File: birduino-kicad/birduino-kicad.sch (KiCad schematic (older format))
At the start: 28 parts, among them J1 Conn_01x03_Male, J10 Conn_01x01_Male, J2 Conn_01x02_Male, J3 Conn_02x05_Odd_Even, J4 Conn_01x04, J5 Conn_01x01_Male, J6 Conn_01x01_Male, J7 Conn_01x01_Male, J8 Conn_02x02_Odd_Even, J9 Conn_01x02, Q1 2N7000, Q2 2N7000, Q3 2N7000, SW1 SW_Push_Dual, SW2 SW_Push_Dual, SW3 SW_Push_Dual, SW4 SW_Push_Dual, U1 ATMEGA328-PU, U2 DS18B20

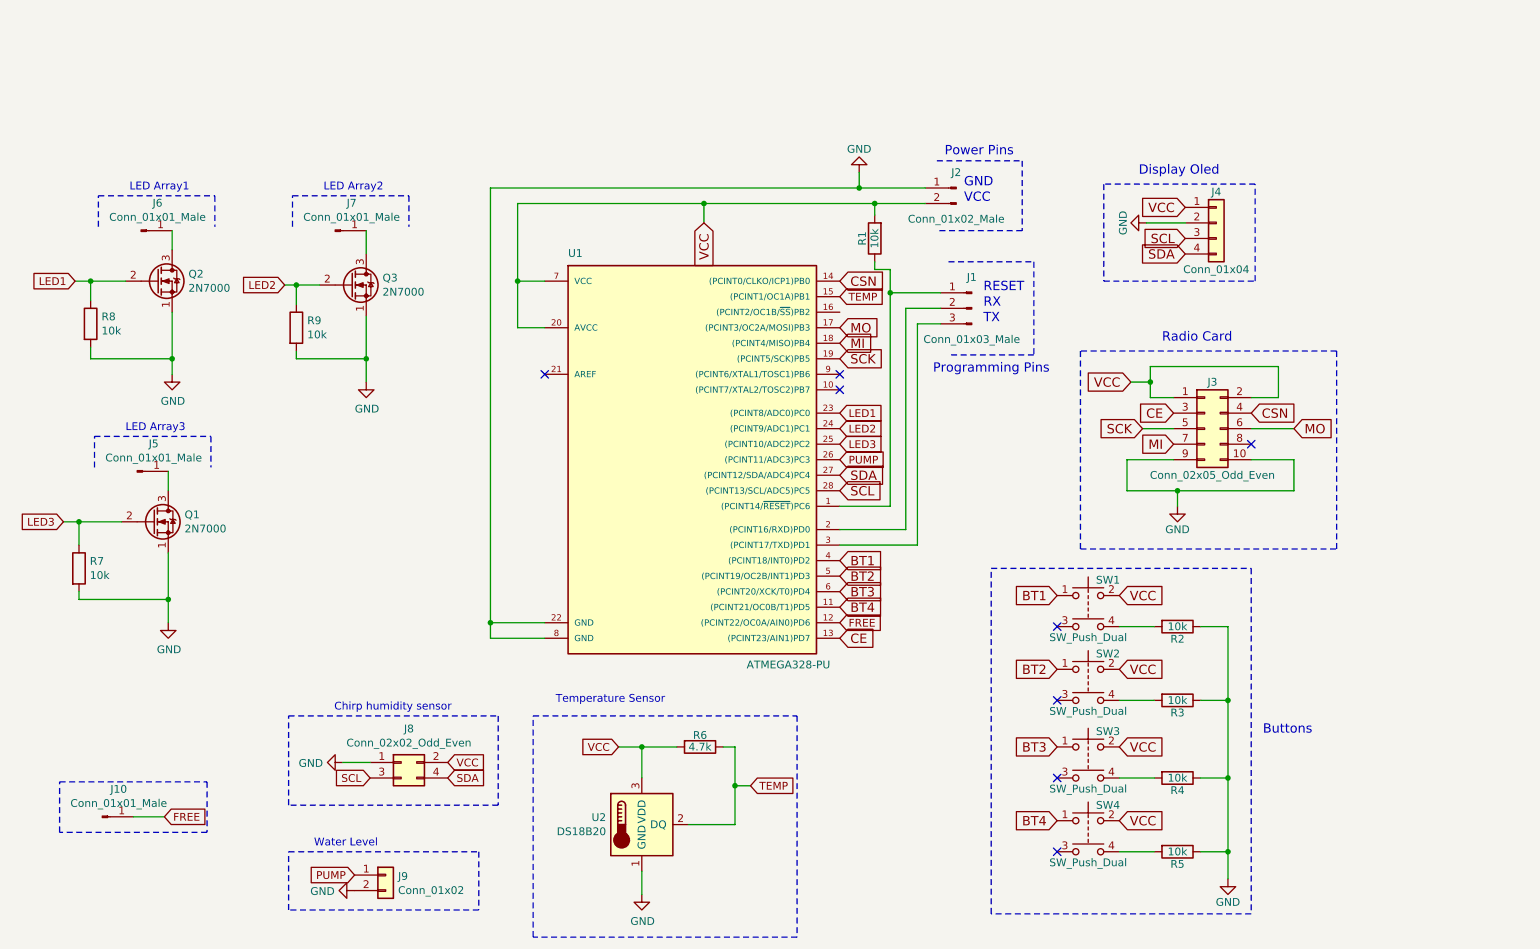
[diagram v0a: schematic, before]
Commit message: feat: First final version 1.0. 3D image added to readme
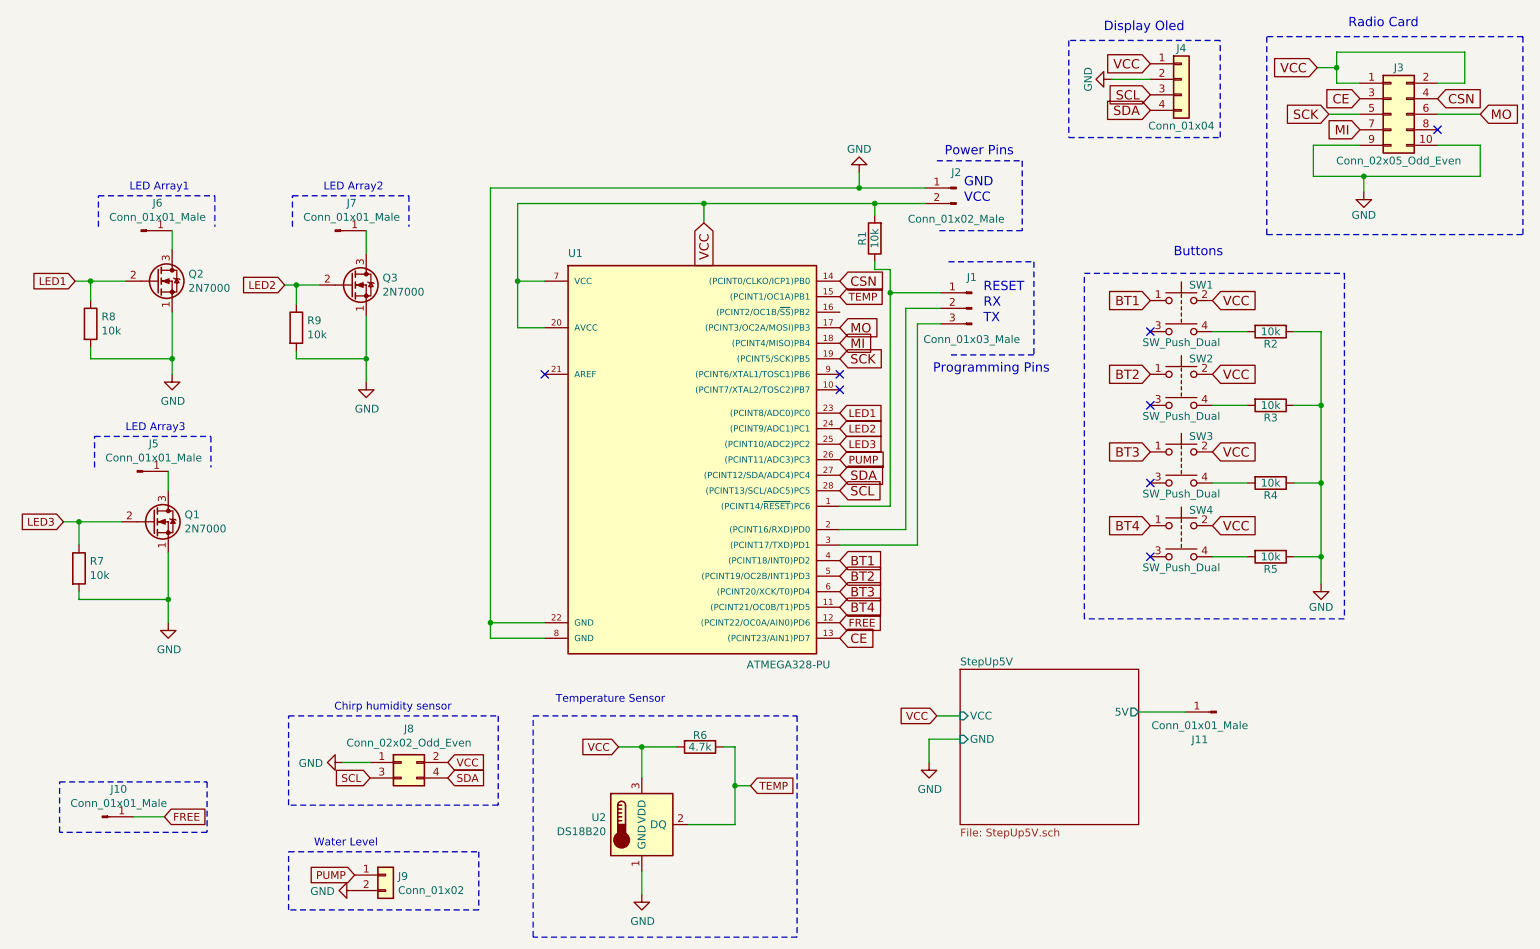
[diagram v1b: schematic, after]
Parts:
- added J11: Conn_01x01_Male, Connector_PinHeader_2.54mm:PinHeader_1x01_P2.54mm_Vertical, symbol Connector:Conn_01x01_Male
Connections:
- new net StepUp5V/5V: J11.1 (Pin_1)
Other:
- moved on the sheet: J3, J4, R2, R3, R4, R5, SW1, SW2, SW3, SW4
